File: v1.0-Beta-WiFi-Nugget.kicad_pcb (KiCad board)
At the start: 2 copper layers, 36 x 50 mm, 54 parts, among them J1 Micro USB, J2 JST PH 2.0, J3 JST_SH_SM03B-SRSS-TB_1x03-1MP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, Q1 UMH3N, Q2 DMG3415, SW1 SPDT, SW2 UP, SW3 Reset, SW4 DOWN, SW5 LEFT, SW6 RIGHT, U1 CP2102N-A01-GQFN24, U2 SH1106, U3 MCP73831-2-OT, U4 ESP-12F, U5 AP2112K-3.3

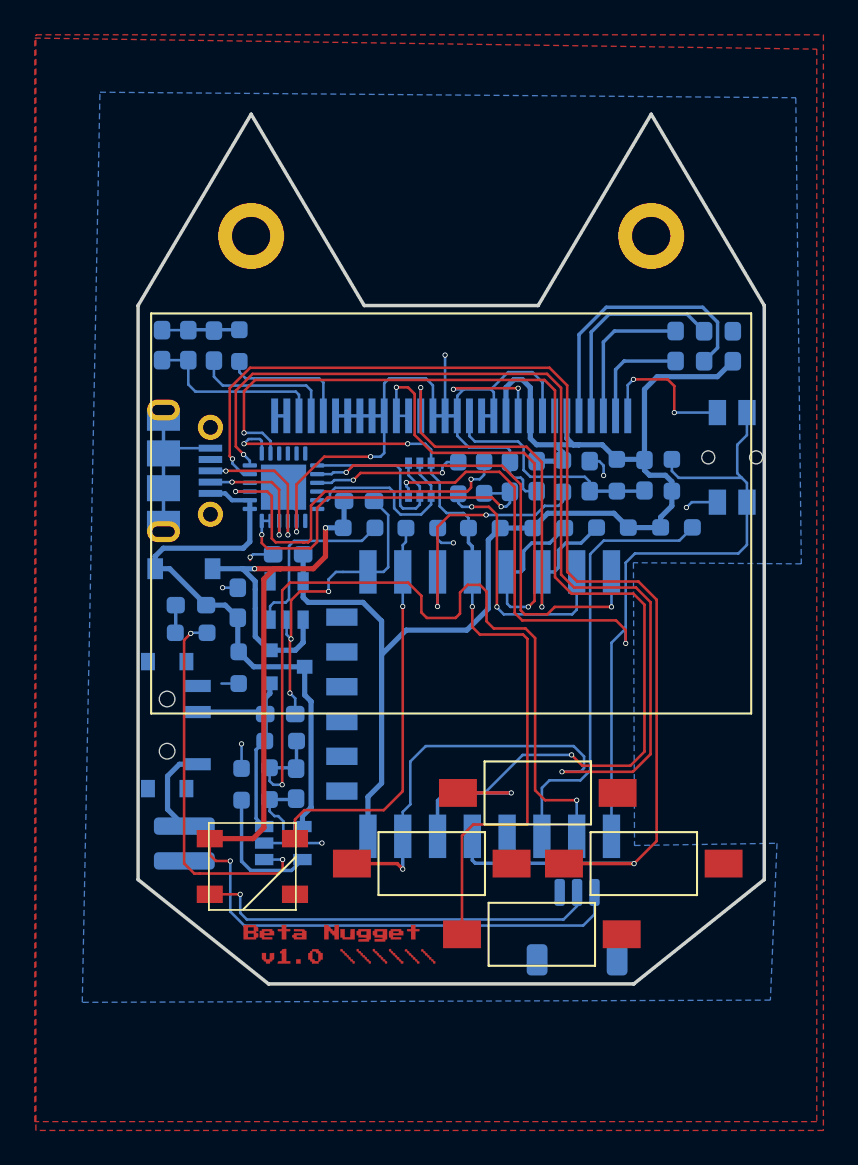
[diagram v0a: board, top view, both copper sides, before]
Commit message: v1.0 board file update
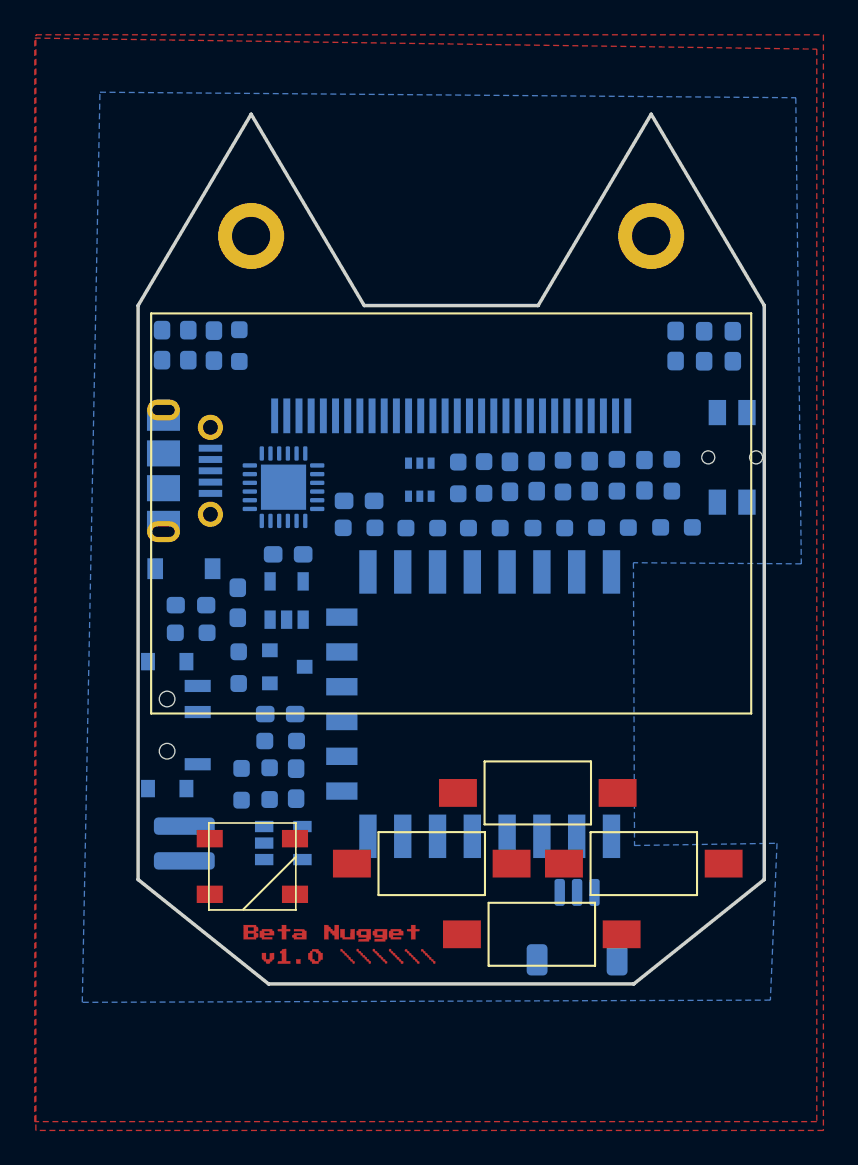
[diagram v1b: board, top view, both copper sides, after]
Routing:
- net GNDREF: track 113.2 -> 0.00 mm, vias 17 -> 0
- net GPIO13: track 76.9 -> 0.00 mm, vias 3 -> 0
- net +3V3: track 75.6 -> 0.00 mm
- net GPIO14: track 73.0 -> 0.00 mm, vias 2 -> 0
- net GPIO12: track 68.4 -> 0.00 mm, vias 3 -> 0
- net VMAX: track 67.7 -> 0.00 mm, vias 3 -> 0
- net ESP_RST: track 59.8 -> 0.00 mm, vias 2 -> 0
- net A0: track 49.2 -> 0.00 mm, vias 2 -> 0
- net GPIO0: track 48.4 -> 0.00 mm, vias 3 -> 0
- net VBUS: track 32.8 -> 0.00 mm
- net SDA: track 29.9 -> 0.00 mm, vias 2 -> 0
- net TXD: track 27.1 -> 0.00 mm, vias 2 -> 0
- net SCL: track 27.0 -> 0.00 mm, vias 2 -> 0
- net Net-(R10-Pad2): track 24.9 -> 0.00 mm
- net DOUT: track 23.4 -> 0.00 mm, vias 1 -> 0
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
